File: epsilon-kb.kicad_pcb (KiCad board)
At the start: 2 copper layers, 3.4 x 3 mm, 35 parts, among them J1 OLED-128x64, J2 OLED-128x32, SW1 SW_Push, SW10 SW_Push, SW11 SW_SPDT, SW2 SW_Push, SW3 SW_Push, SW4 SW_Push, SW5 SW_Push, SW6 SW_Push, SW7 SW_Push, SW8 SW_Push, SW9 SW_Push, U1 xiao-ble

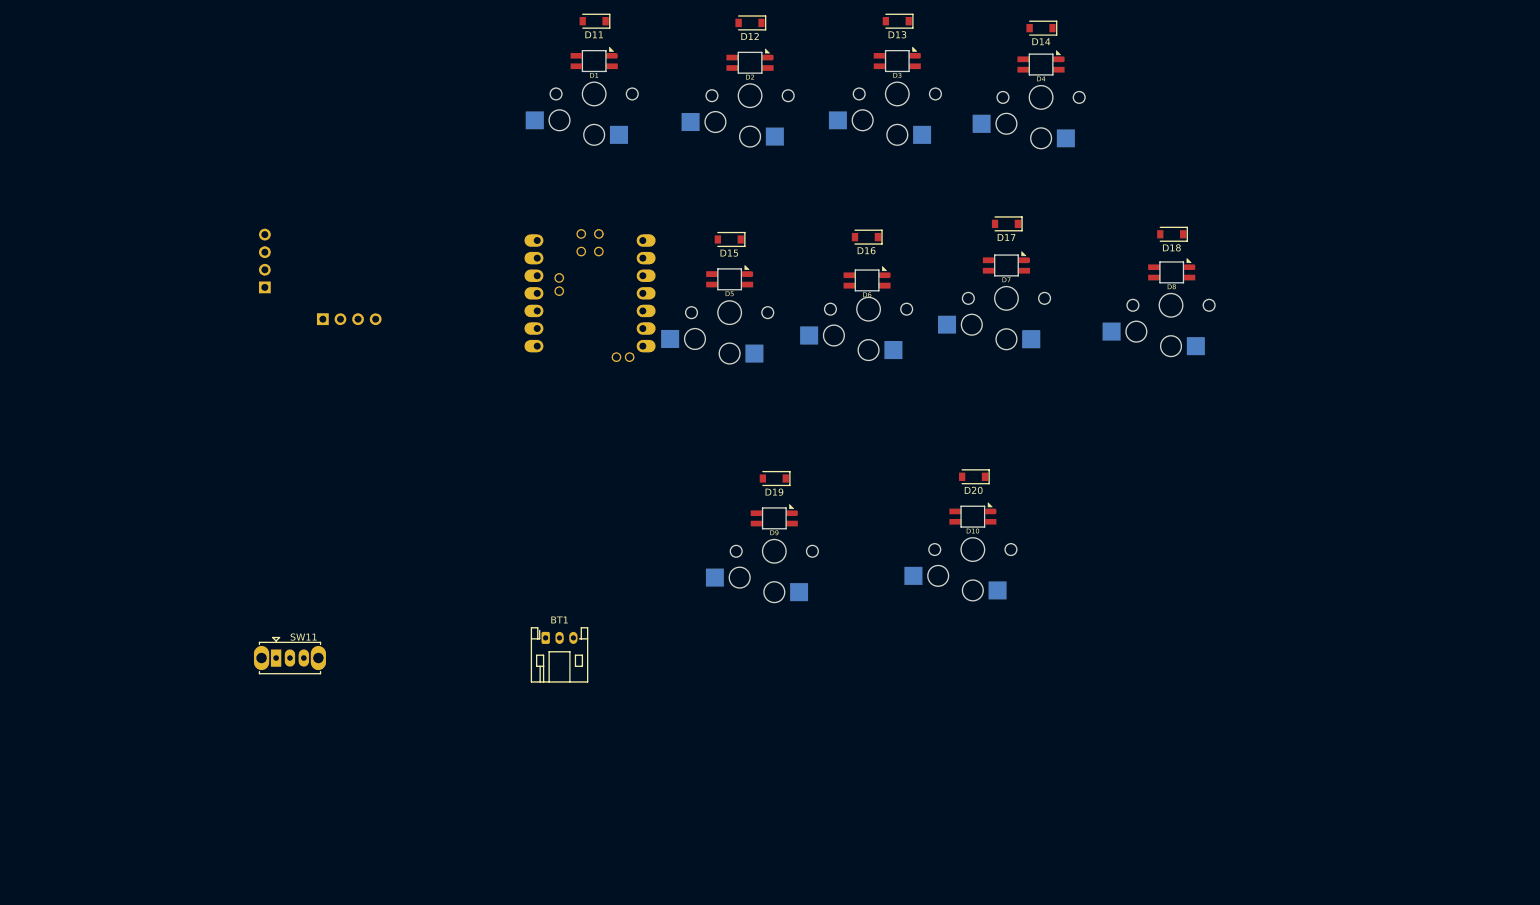
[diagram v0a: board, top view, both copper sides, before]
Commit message: PCB
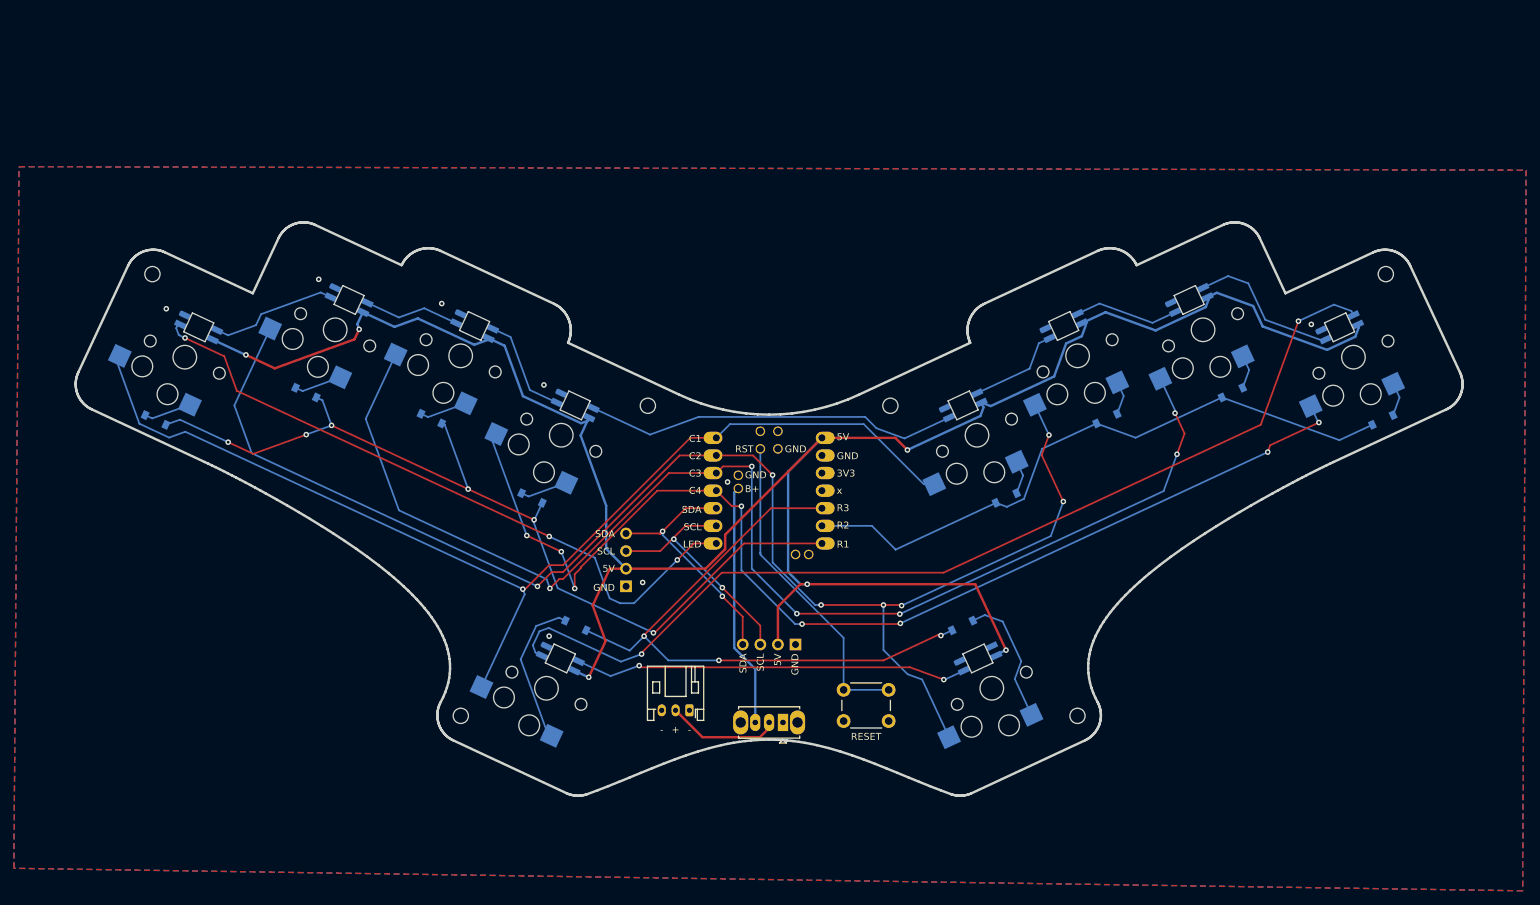
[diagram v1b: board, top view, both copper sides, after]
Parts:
- added REF**: MountingHole_2.2mm_M2, MountingHole:MountingHole_2.2mm_M2, F.Cu at (132.5, 81.2)
- added REF**: MountingHole_2.2mm_M2, MountingHole:MountingHole_2.2mm_M2, F.Cu at (194.5, 126.0)
- added REF**: MountingHole_2.2mm_M2, MountingHole:MountingHole_2.2mm_M2, F.Cu at (105.5, 126.0)
- added REF**: MountingHole_2.2mm_M2, MountingHole:MountingHole_2.2mm_M2, F.Cu at (167.5, 81.2)
- added REF**: MountingHole_2.2mm_M2, MountingHole:MountingHole_2.2mm_M2, F.Cu at (239.0, 62.2)
- added REF**: MountingHole_2.2mm_M2, MountingHole:MountingHole_2.2mm_M2, F.Cu at (61.0, 62.2)
- added SW12: SW_Push, Button_Switch_THT:SW_PUSH_6mm, F.Cu at (160.8, 122.3)
- D1, D10, D2, D3, D4, D5, D6, D7, D8, D9: value SK6812MINI -> SK6812MINI-E; moved to B.Cu
- D11, D12, D13, D14, D15, D16, D17, D18, D19, D20: moved to B.Cu
- moved D14 100.0 mm to (115.8, 94.6), turned to 155 degrees
- moved D13 88.4 mm to (101.3, 83.1), turned to 155 degrees
- moved D11 85.6 mm to (61.4, 83.3), turned to 155 degrees
- moved SW4 84.7 mm to (120.0, 85.5), turned to 155 degrees
- moved D12 83.4 mm to (83.1, 79.3), turned to 155 degrees
- moved D4 83.3 mm to (122.0, 81.2), turned to 155 degrees
- moved J1 76.7 mm to (150.0, 115.7), turned to 180 degrees
- moved SW11 73.7 mm to (152.0, 127.0), turned to 180 degrees
- moved SW3 73.5 mm to (105.5, 74.0), turned to 155 degrees
- moved D3 72.0 mm to (107.5, 69.7), turned to 155 degrees
- moved SW1 70.2 mm to (65.7, 74.2), turned to 155 degrees
- moved D1 68.8 mm to (67.7, 69.9), turned to 155 degrees
- moved SW2 68.8 mm to (87.4, 70.3), turned to 155 degrees
- moved J2 67.7 mm to (127.8, 97.5)
- moved D2 67.2 mm to (89.4, 66.0), turned to 155 degrees
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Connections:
- D1 pad 1: Net-(D2-Pad3) -> +5V
- D1 pad 2: GND -> Net-(D1-Pad2)
- D1 pad 3: /LED_IN -> GND
- D1 pad 4: +5V -> /LED_IN
- D10 pad 1: /LED_OUT -> +5V
- D10 pad 2: GND -> /LED_OUT
- D10 pad 3: Net-(D10-Pad3) -> GND
- D10 pad 4: +5V -> Net-(D10-Pad4)
- D2 pad 1: Net-(D3-Pad3) -> +5V
- D2 pad 2: GND -> Net-(D2-Pad2)
- D2 pad 3: Net-(D2-Pad3) -> GND
- D2 pad 4: +5V -> Net-(D1-Pad2)
- D3 pad 1: Net-(D4-Pad3) -> +5V
- D3 pad 2: GND -> Net-(D3-Pad2)
- D3 pad 3: Net-(D3-Pad3) -> GND
- D3 pad 4: +5V -> Net-(D2-Pad2)
- D4 pad 1: Net-(D5-Pad3) -> +5V
- D4 pad 2: GND -> Net-(D4-Pad2)
- D4 pad 3: Net-(D4-Pad3) -> GND
- D4 pad 4: +5V -> Net-(D3-Pad2)
- D5 pad 1: Net-(D5-Pad1) -> +5V
- D5 pad 2: GND -> Net-(D5-Pad2)
- D5 pad 3: Net-(D5-Pad3) -> GND
- D5 pad 4: +5V -> Net-(D4-Pad2)
- D6 pad 1: Net-(D6-Pad1) -> +5V
- D6 pad 2: GND -> Net-(D6-Pad2)
- D6 pad 3: Net-(D5-Pad1) -> GND
- D6 pad 4: +5V -> Net-(D5-Pad2)
- D7 pad 1: Net-(D8-Pad3) -> +5V
- D7 pad 2: GND -> Net-(D7-Pad2)
- D7 pad 3: Net-(D6-Pad1) -> GND
- D7 pad 4: +5V -> Net-(D6-Pad2)
- D8 pad 1: Net-(D9-Pad3) -> +5V
- D8 pad 2: GND -> Net-(D8-Pad2)
- D8 pad 3: Net-(D8-Pad3) -> GND
- D8 pad 4: +5V -> Net-(D7-Pad2)
- D9 pad 1: Net-(D10-Pad3) -> +5V
- D9 pad 2: GND -> Net-(D10-Pad4)
- D9 pad 3: Net-(D9-Pad3) -> GND
- D9 pad 4: +5V -> Net-(D8-Pad2)
- U1 pad 17: unconnected-(U1-Pad17) -> /RST
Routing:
- net +5V: track 0.00 -> 318.1 mm, vias 0 -> 6
- net C2: track 0.00 -> 208.9 mm, vias 0 -> 7
- net C3: track 0.00 -> 184.1 mm, vias 0 -> 6
- net C4: track 0.00 -> 164.4 mm, vias 0 -> 8
- net C1: track 0.00 -> 160.2 mm, vias 0 -> 1
- net Net-(D8-Pad2): track 0.00 -> 144.4 mm, vias 0 -> 2
- net R1: track 0.00 -> 131.2 mm, vias 0 -> 6
- net /LED_IN: track 0.00 -> 96.9 mm, vias 0 -> 3
- net R2: track 0.00 -> 91.8 mm
- net R3: track 0.00 -> 90.2 mm, vias 0 -> 3
- net Net-(D10-Pad4): track 0.00 -> 57.5 mm, vias 0 -> 2
- net Net-(D4-Pad2): track 0.00 -> 54.3 mm
- net /RST: track 0.00 -> 46.3 mm
- net /SDA: track 0.00 -> 35.7 mm, vias 0 -> 2
- net +BATT: track 0.00 -> 35.3 mm
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- added copper zone on B.Cu, net GND
- added copper zone on F.Cu, net GND
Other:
- board size 3.4 x 3 mm -> 200.2 x 82.7 mm
- board text added: "+"
- board text added: "-"
- board text added: "3V3"
- board text added: "5V"
- board text added: "B+"
- board text added: "C1"
- board text added: "C2"
- board text added: "C3"
- board text added: "C4"
- board text added: "Epsilon by DeltaWhy version ${pcbVersion} https://github.com/DeltaWhy/epsilon-kb"
- board text added: "GND"
- board text added: "JLCJLCJLCJLC"
- board text added: "LED"
- board text added: "R1"
- board text added: "R2"
- board text added: "R3"
- board text added: "RESET"
- board text added: "RST"
- board text added: "SCL"
- board text added: "SDA"
- board text added: "x"
